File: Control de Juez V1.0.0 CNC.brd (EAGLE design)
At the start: 35.5 x 58.4 mm, 31 parts, among them IC1 MEGA48/88/168-AU, Q1 MMBT3904, Q2 MMBT3904, Q3 MMBT3904, SW1 JS202011CQN, SW2 3-1825910-1, SW3 3-1825910-1, SW4 3-1825910-1

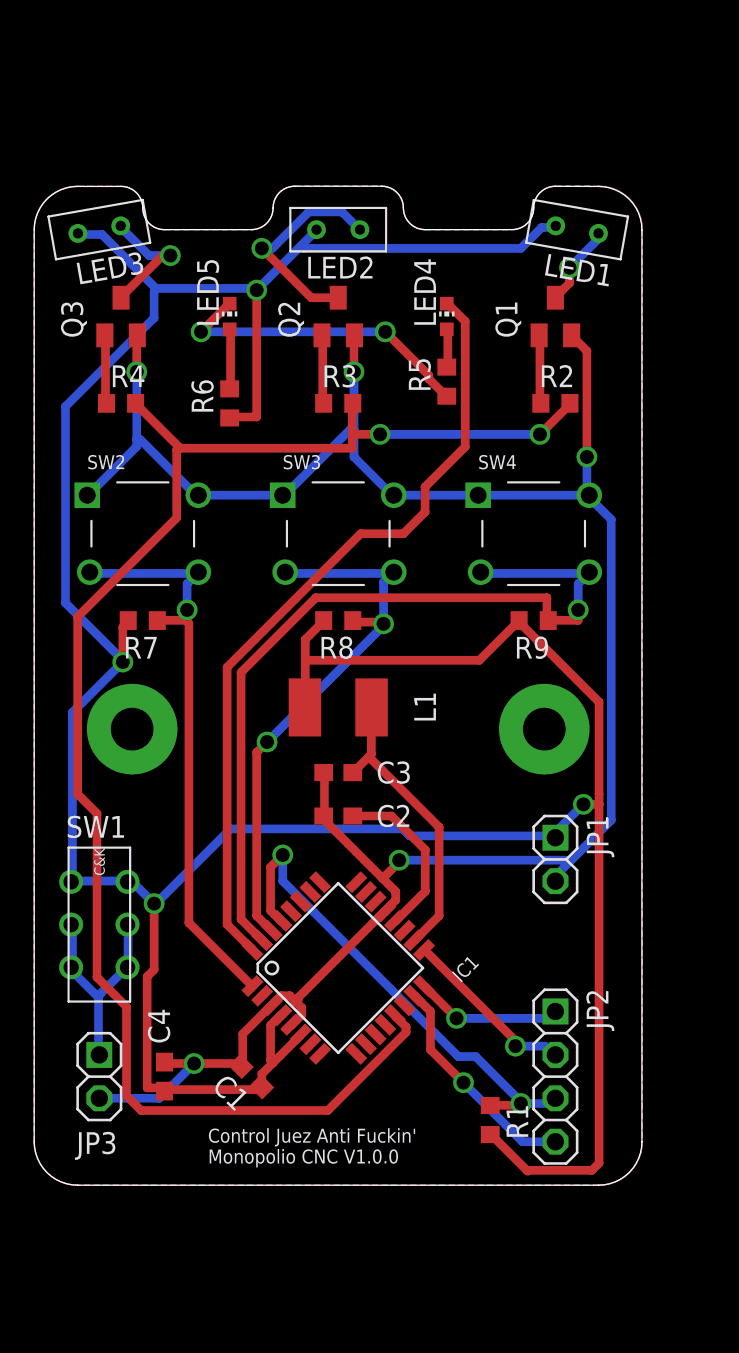
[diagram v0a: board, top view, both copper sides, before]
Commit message: Add files via upload
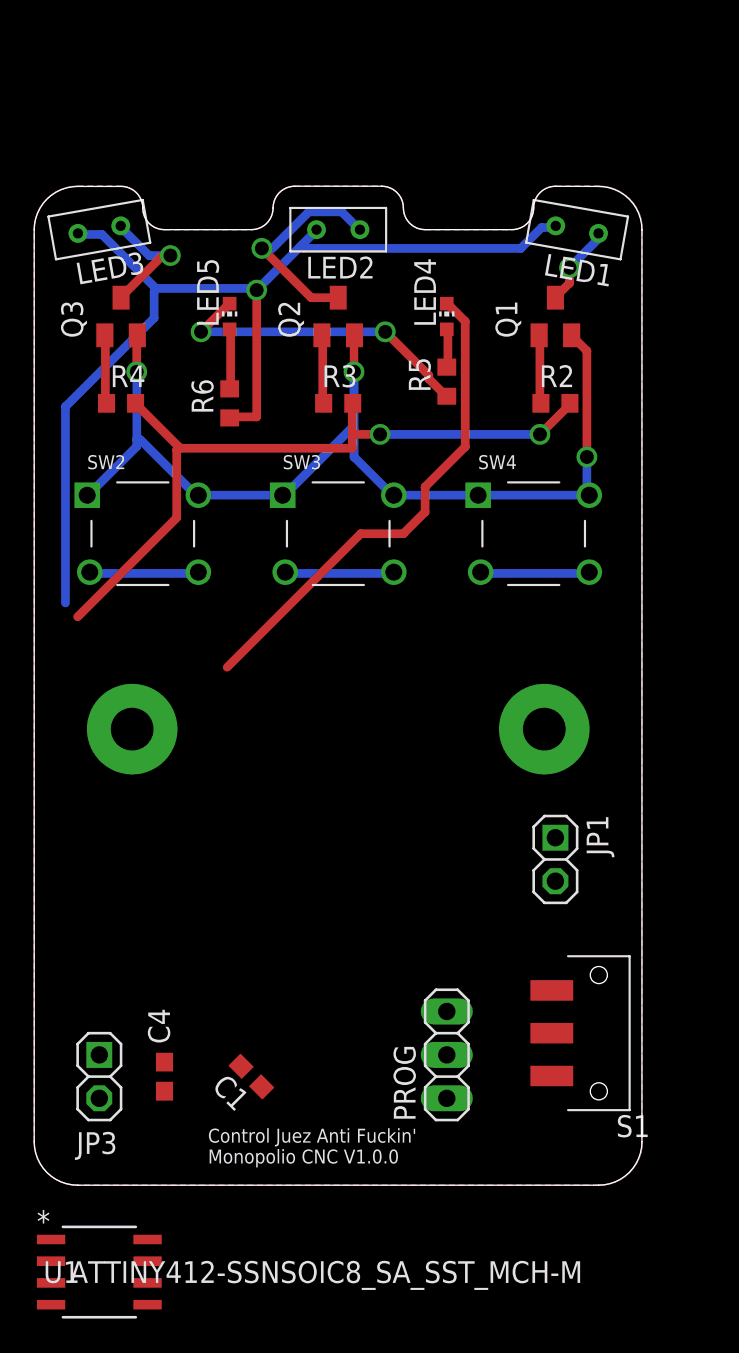
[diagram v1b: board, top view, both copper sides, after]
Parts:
- removed C2, C3: 0.1uF, rcl:C0603
- removed IC1: MEGA48/88/168-AU, avr-8:TQFP32-08
- removed JP2: (no value), pinhead-2:1X04-S
- removed L1: 10uH, rcl:L1812
- removed R1, R7, R8, R9: 10K, rcl:R0603
- removed SW1: JS202011CQN, C&K-Slider_Switch:PTH
- added PROG: (no value), pinhead:1X03
- added S1: JS102011SAQN, JS102011SAQN:SW_JS102011SAQN
- added U1: ATTINY412-SSNSOIC8_SA_SST_MCH-M, attiny412:SOIC8_SA_SST_MCH-M
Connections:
- removed net N$2: C3.1, IC1.18, L1.1
- removed net N$3: C2.1, IC1.20
- removed net N$4: IC1.16, JP2.1
- removed net N$5: IC1.17, JP2.2
- removed net N$6: JP3.1, SW1.1.1, SW1.1.2, SW1.2.1, SW1.2.2
- removed net RESET: IC1.29, JP2.3, R1.1
- new net BAT+: JP3.1, S1.2, S1.3
- net +5V: now also PROG.1, S1.1, U1.1; no longer IC1.4, IC1.6, L1.2, R1.2, R7.2, R8.2, R9.2, SW1.3.1, SW1.3.2
- net GND: now also PROG.3, U1.8; no longer C2.2, C3.2, IC1.21, IC1.3, IC1.5
- net GO: now also U1.3; no longer IC1.31, R9.1
- net LEDS: now also U1.5; no longer IC1.13
- net LEDSMD: now also U1.4; no longer IC1.32
- net N$1: now also PROG.2, U1.6; no longer IC1.15, JP2.4
- net READY: now also U1.2; no longer IC1.1, R7.1
- net RST: now also U1.7; no longer IC1.30, R8.1
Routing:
- net +5V: track 203.4 -> 62.7 mm, vias 4 -> 1
- net GND: track 130.3 -> 58.4 mm, vias 5 -> 3
- net LEDS: track 91.3 -> 42.3 mm
- net GO: track 48.5 -> 6.50 mm, vias 1 -> 0
- net RESET: track 29.4 -> 0.00 mm, vias 2 -> 0
- net READY: track 34.2 -> 6.51 mm, vias 1 -> 0
- net RST: track 33.0 -> 6.51 mm, vias 2 -> 0
- net N$2: track 17.3 -> 0.00 mm
- net LEDSMD: track 46.1 -> 29.0 mm
- net N$6: track 13.3 -> 0.00 mm
- net N$1: track 13.1 -> 0.00 mm, vias 1 -> 0
- net N$5: track 10.4 -> 0.00 mm, vias 1 -> 0
- net N$3: track 10.1 -> 0.00 mm
- net N$4: track 8.63 -> 0.00 mm, vias 1 -> 0

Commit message: Add files via upload
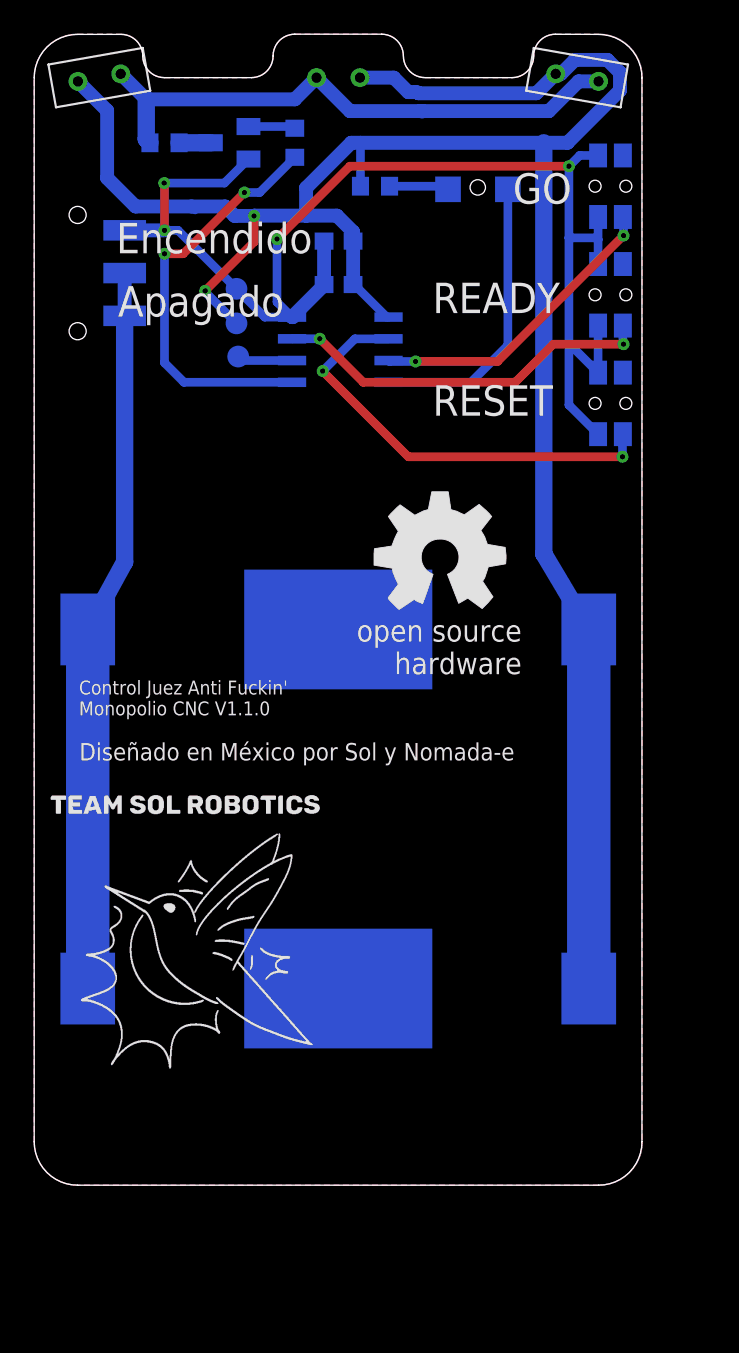
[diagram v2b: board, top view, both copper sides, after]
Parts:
- removed JP1, JP3: (no value), pinhead-2:1X02-S
- removed LED4: (no value), led:CHIP-LED0603
- removed PROG: (no value), pinhead:1X03
- removed Q2, Q3: MMBT3904, FAIRCHILD-MMBT3904_Transistor:SOT23
- removed R3, R4: 1K, rcl:R0603
- removed R5: 330E, rcl:R0603
- removed SW2, SW3, SW4: 3-1825910-1, TE-Push_button:TE_3-1825910-1
- added BT2: BU2032SM-HD-G, BU2032SM-HD-G:BAT_BU2032SM-HD-G
- added GND, UPDI, V+: TPB1,27, testpad:B1,27
- added GO, READY, RESET: EVQ-P7L01P, EVQ-P7L01P:SW_EVQ-P7L01P
- added GOLD_ORB_SM1: OSHWLOGOLOGO8MM, oshw:OSHW_8MM
- added R1: 1K, rcl:R0603
- BT1: value HOLD-BATTERY-3-AAA -> BU2032SM-HD-G; device BATTERY_HOLDER_3AAA-C9091:HOLDER-3-AAA -> BU2032SM-HD-G:BAT_BU2032SM-HD-G
- LED5: device led:CHIP-LED0603 -> led:SML1206
- R6: value 330E -> 1k
- moved U1 55.7 mm to (17.9, 48.9), flipped to the bottom
- moved S1 53.9 mm to (2.54, 53.3), flipped to the bottom
- moved C4 49.9 mm to (17.8, 55.2), flipped to the bottom, turned to 0 degrees
- moved C1 46.6 mm to (17.8, 52.7), flipped to the bottom, turned to 0 degrees
- moved Q1 21.6 mm to (11.4, 61.0), flipped to the bottom, turned to 270 degrees
- moved R2 21.6 mm to (15.2, 61.0), flipped to the bottom, turned to 270 degrees
- moved LED5 16.3 mm to (25.9, 58.2), flipped to the bottom
- moved R6 15.3 mm to (19.9, 58.4), flipped to the bottom, turned to 180 degrees
- moved BT1 15.2 mm to (17.8, 11.5), flipped to the bottom
- moved LED1 8.89 mm to (31.8, 64.8)
- moved LED2 8.89 mm to (17.8, 64.8), flipped to the bottom
- moved LED3 8.89 mm to (3.81, 64.8)
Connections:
- removed net BAT+: JP3.1, S1.2, S1.3
- removed net N$10: Q3.B, R4.1
- removed net N$11: Q2.B, R3.1
- removed net N$13: LED5.C, R5.1
- removed net N$15: LED4.A, R5.2
- removed net N$7: LED1.2, Q1.C
- removed net N$8: LED2.2, Q2.C
- removed net N$9: LED3.2, Q3.C
- new net N$2: BT1.-, BT2.-, S1.1, S1.2
- new net N$3: LED1.2, LED2.2, LED3.2, R1.1
- new net N$4: Q1.C, R1.2
- net +5V: now also BT1.+, BT2.+, V+.TP; no longer JP1.1, PROG.1, S1.1
- net GND: now also GND.TP, GO.1_1, GO.1_2, READY.1_1, READY.1_2, RESET.1_1, RESET.1_2, S1.3; no longer JP1.2, JP3.2, PROG.3, Q2.E, Q3.E, SW2.1, SW2.2, SW3.1, SW3.2, SW4.1, SW4.2
- net GO: now also GO.2_1, GO.2_2; no longer SW4.3, SW4.4
- net LEDS: no longer R3.2, R4.2
- net LEDSMD: now also LED5.C; no longer LED4.C
- net N$1: now also UPDI.TP; no longer PROG.2
- net READY: now also READY.2_1, READY.2_2; no longer SW2.3, SW2.4
- net RST: now also RESET.2_1, RESET.2_2; no longer SW3.3, SW3.4
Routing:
- net +5V: track 62.7 -> 129.4 mm, vias 1 -> 2
- net N$2: track 0.00 -> 42.9 mm
- net N$3: track 0.00 -> 33.3 mm
- net READY: track 6.51 -> 25.6 mm, vias 0 -> 2
- net GND: track 58.4 -> 77.2 mm, vias 3 -> 4
- net N$13: track 18.4 -> 0.00 mm, vias 2 -> 0
- net LEDS: track 42.3 -> 24.3 mm
- net RST: track 6.51 -> 22.5 mm, vias 0 -> 2
- net N$8: track 12.8 -> 0.00 mm, vias 1 -> 0
- net LEDSMD: track 29.0 -> 17.0 mm
- net GO: track 6.50 -> 17.9 mm, vias 0 -> 2
- net N$9: track 7.59 -> 0.00 mm, vias 1 -> 0
- net N$7: track 4.80 -> 0.00 mm, vias 1 -> 0
- net N$10: track 4.03 -> 0.00 mm
- net N$11: track 4.03 -> 0.00 mm
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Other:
- board size 35.5 x 58.4 mm -> 35.5 x 67.3 mm
- board text added: "Apagado"
- board text added: "Control Juez Anti Fuckin' Monopolio CNC V1.1.0"
- board text added: "Diseñado en México por Sol y Nomada-e"
- board text added: "Encendido"
- board text added: "GO"
- board text added: "READY"
- board text added: "RESET"
- board text removed: "Control Juez Anti Fuckin' Monopolio CNC V1.0.0"
